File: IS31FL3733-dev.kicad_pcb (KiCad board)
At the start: 2 copper layers, 39.7 x 61.7 mm, 214 parts, among them J1 Conn_01x11_Female, U1 IS31FL3733-QF

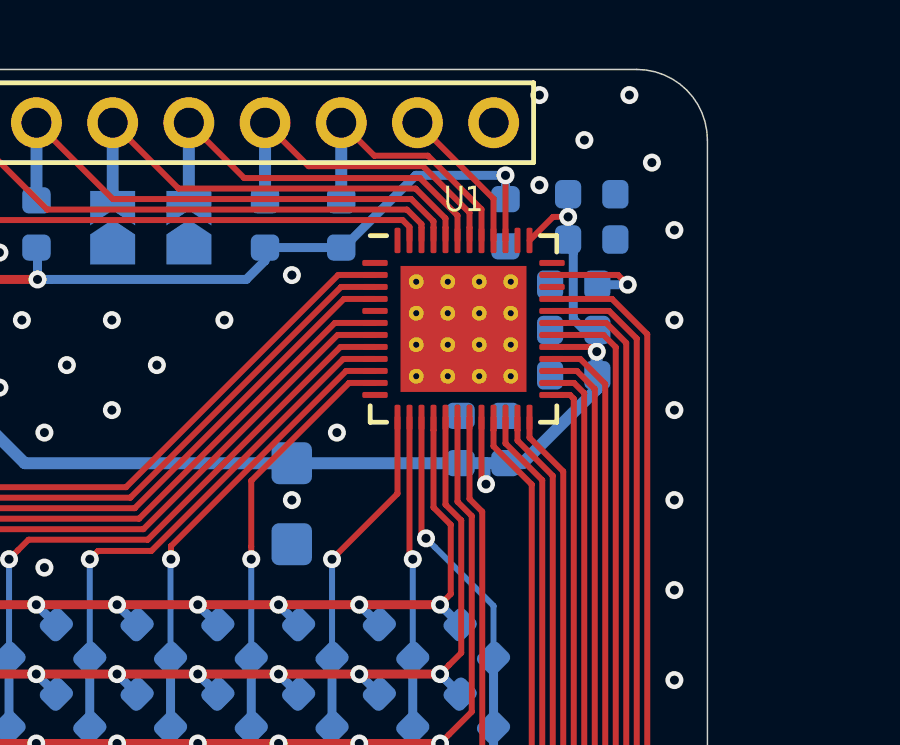
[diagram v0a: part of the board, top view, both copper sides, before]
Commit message: fix problems with the board
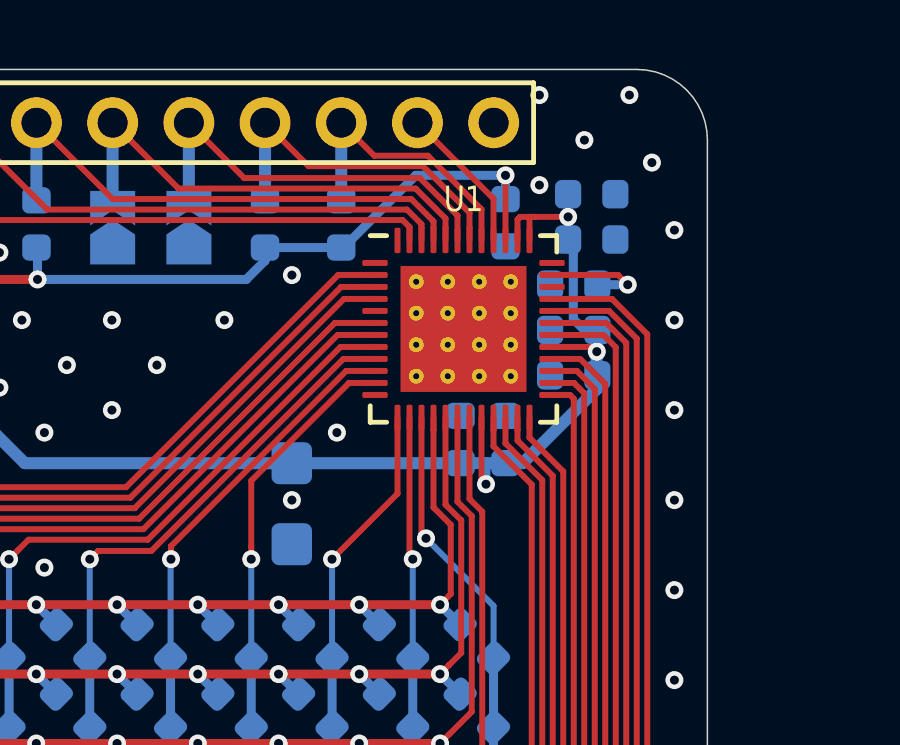
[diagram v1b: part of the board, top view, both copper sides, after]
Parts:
- turned C1 to 90 degrees
- turned C2 to 180 degrees
- turned C3 to 90 degrees
- turned C4 to 0 degrees
- turned C5 to 0 degrees
- turned C6 to 90 degrees
- turned C7 to 180 degrees
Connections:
- C1 pad 1: VCC -> GND
- C1 pad 2: GND -> VCC
- C2 pad 1: GND -> VCC
- C2 pad 2: VCC -> GND
- C3 pad 1: GND -> VCC
- C3 pad 2: VCC -> GND
- C4 pad 1: GND -> VCC
- C4 pad 2: VCC -> GND
- C5 pad 1: GND -> VCC
- C5 pad 2: VCC -> GND
- C6 pad 1: GND -> VCC
- C6 pad 2: VCC -> GND
- C7 pad 1: GND -> VCC
- C7 pad 2: VCC -> GND
- U1 pad 38: GND -> VCC
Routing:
- net VCC: track 46.2 -> 48.0 mm
